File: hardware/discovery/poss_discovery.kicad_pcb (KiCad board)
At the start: 2 copper layers, 96.5 x 66 mm, 118 parts, among them CON1 USB-MICRO-B, SW1 SW_PUSH, SW10 SW_PUSH, SW11 SW_PUSH, SW12 SW_PUSH, SW13 SW_PUSH, SW14 SW_PUSH, SW15 SW_PUSH, SW16 SW_PUSH, SW18 SW_PUSH, SW19 SW_PUSH, SW2 SW_PUSH, SW20 SW_PUSH, SW21 SW_PUSH, SW22 SW_PUSH, SW3 SW_PUSH, SW4 SW_PUSH, SW5 SW_PUSH, SW6 SW_PUSH, SW7 SW_PUSH, SW8 SW_PUSH, SW9 SW_PUSH, U10 STM32_SWD_Connector, U2 MCP73831, U3 BD33IA5, U4 STM32F407VG, U5 SGTL5000, U6 encoder_and_switch, U7 encoder_and_switch, U8 MOLEX_microSD_47219-2001, U9 SSD1306, X1 CRYSTAL

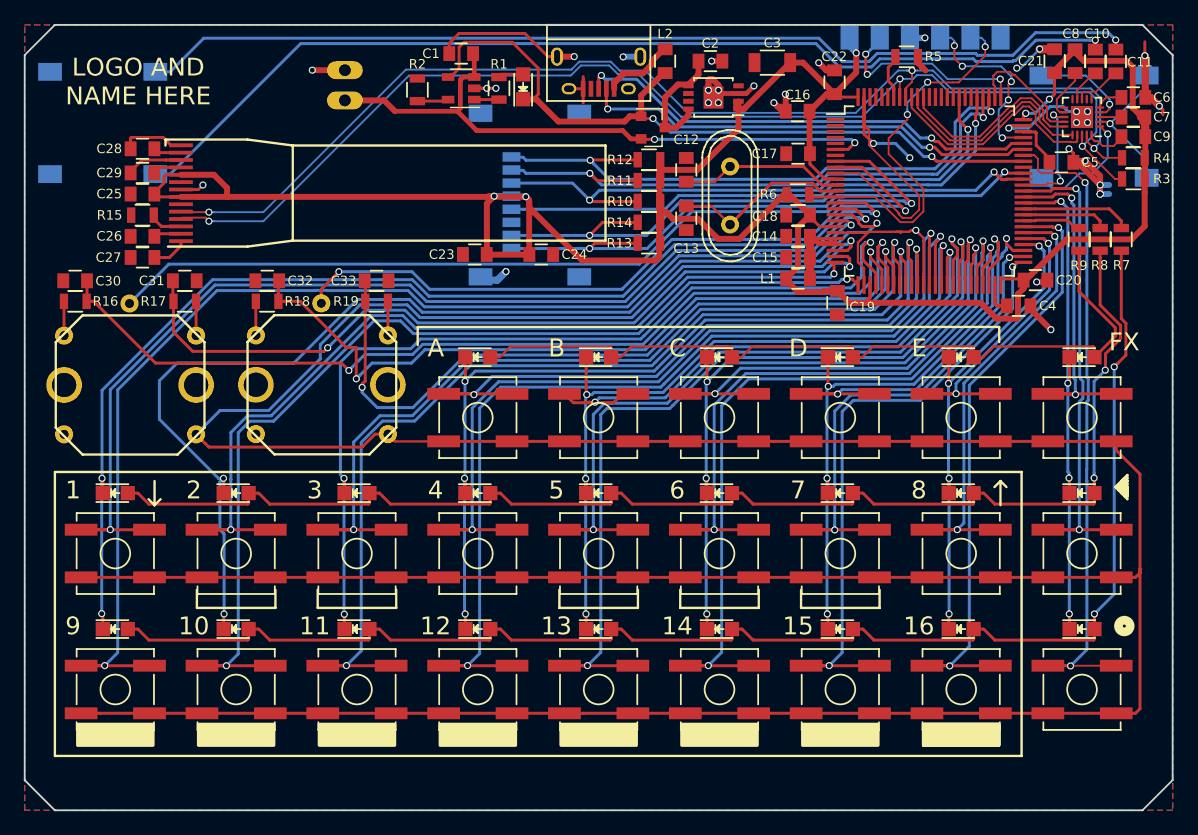
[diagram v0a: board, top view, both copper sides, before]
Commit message: Discovery: Restart from RevA
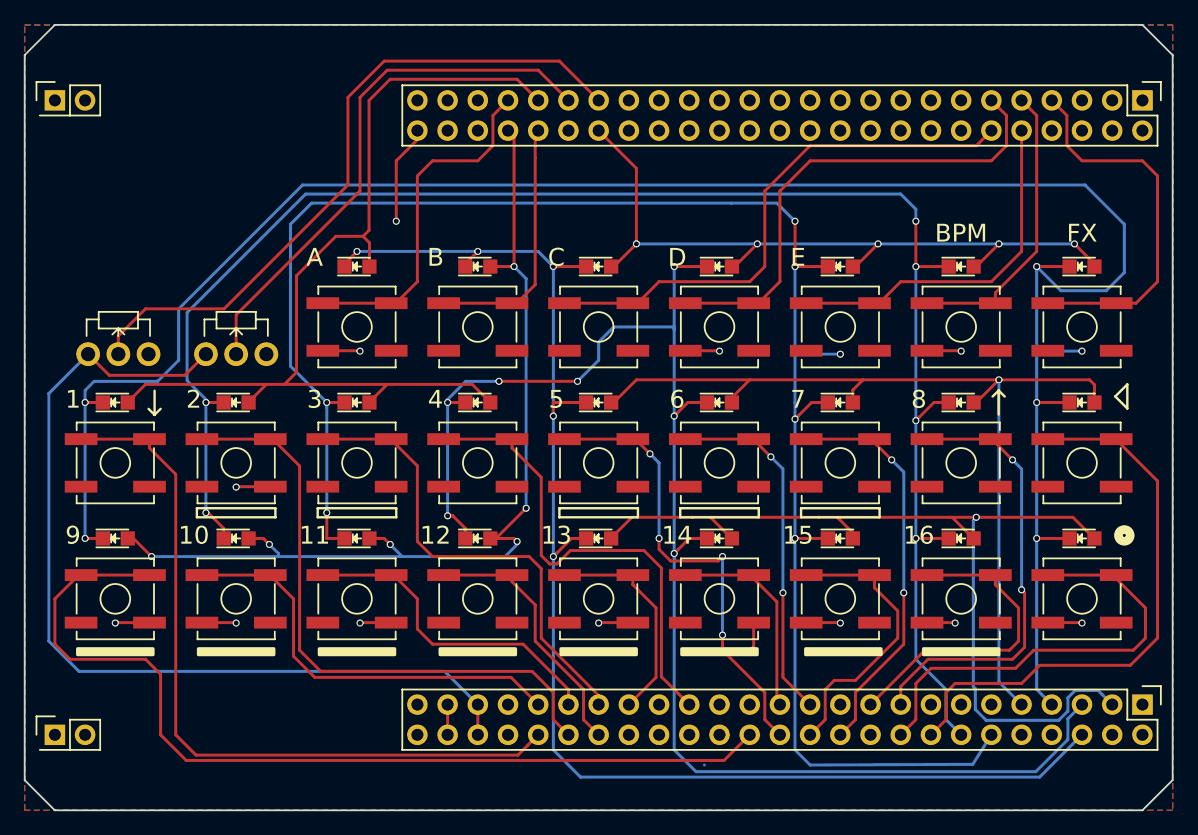
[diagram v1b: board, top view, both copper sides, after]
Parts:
- removed BAT1: LED, LEDs:LED_0805
- removed BT1: BATTERY, Connect:PINHEAD1-2
- removed C1, C25, C26, C27: 10uF, Capacitors_SMD:C_0805
- removed C10, C11, C14, C28, C29: 1uF, Capacitors_SMD:C_0805
- removed C12, C13: C, Capacitors_SMD:C_0805
- removed C15, C17, C18, C19, C20, C21, C22, C23, C6, C7, C8, C9: 0.1uF, Capacitors_SMD:C_0805
- removed C16, C24: 22uF, Capacitors_SMD:C_0805
- removed C2: 4.7uF, Capacitors_SMD:C_0805
- removed C3: 47uF, Capacitors_SMD:C_1206
- removed C30, C31, C32, C33: 0,1uF, Capacitors_SMD:C_0805
- removed C4, C5: 2.2uF, Capacitors_SMD:C_0805
- removed CON1: USB-MICRO-B, Connect:USB_Micro-B
- removed D27: DOUBLE_SCH_KCOM_PMEG2005CT, TO_SOT_Packages_SMD:SOT-23
- removed HP_OUT1, LINE_IN1: 3.5_audio_jack, stm32f4-disco:lumberg_3.5_audio_jack_1503_02
- removed L1, L2: 15Ohm, Capacitors_SMD:C_0805
- removed R1: 1K, Resistors_SMD:R_0805
- removed R10, R11, R12, R13, R14, R2, R3, R4, R5, R6: 10K, Resistors_SMD:R_0805
- removed R15, R7, R8, R9: R, Resistors_SMD:R_0805
- removed R16, R17, R18, R19: 27K, Resistors_SMD:R_0805
- removed U10: STM32_SWD_Connector, stm32f4-disco:STM32_SWD_Connector_SMD
- removed U2: MCP73831, TO_SOT_Packages_SMD:SOT-23-5
- removed U3: BD33IA5, Housings_SSOP:MSOP-8-1EP_3x3mm_Pitch0.65mm
- removed U4: STM32F407VG, Housings_QFP:LQFP-100_14x14mm_Pitch0.5mm
- removed U5: SGTL5000, Housings_DFN_QFN:UQFN-20-1EP_3x3mm_Pitch0.4mm
- removed U6, U7: encoder_and_switch, stm32f4-disco:encoder_EC12D
- removed U8: MOLEX_microSD_47219-2001, stm32f4-disco:MOLEX_microSD_47219-2001
- removed U9: SSD1306, stm32f4-disco:MIDAS_MCOT096016AV_OLED
- removed X1: CRYSTAL, Crystals:Crystal_HC49-U_Vertical
- added D19: LED, LEDs:LED_0805, F.Cu at (97.8, 110.5)
- added J1: HEADER_2, Pin_Headers:Pin_Header_Straight_2x01, F.Cu at (82.5, 85.1)
- added J2: HEADER_25x2, Pin_Headers:Pin_Header_Straight_2x25, F.Cu at (174.0, 85.1)
- added J3: HEADER_25x2, Pin_Headers:Pin_Header_Straight_2x25, F.Cu at (174.0, 135.9)
- added J5: HEADER_2, Pin_Headers:Pin_Header_Straight_2x01, F.Cu at (82.5, 138.4)
- added RV1: POT, Potentiometers:Potentiometer_WirePads_Small, F.Cu at (95.2, 106.4)
- added RV2: POT, Potentiometers:Potentiometer_WirePads_Small, F.Cu at (85.3, 106.4)
- added SW17: SW_PUSH, Buttons_Switches_SMD:SW_SPST_B3SL-1002P, F.Cu at (108.0, 104.1)
- moved D25 82.7 mm to (87.6, 121.9)
- moved D10 81.6 mm to (168.9, 110.5)
- moved D24 62.8 mm to (97.8, 121.9)
- moved D18 61.4 mm to (108.0, 110.5)
- moved D16 44.9 mm to (108.0, 99.1)
- moved D23 43.4 mm to (108.0, 121.9)
- moved D1 41.3 mm to (128.3, 121.9)
- moved D17 41.3 mm to (118.1, 110.5)
- moved D2 41.3 mm to (138.4, 121.9)
- moved D3 41.3 mm to (148.6, 121.9)
- moved D4 41.3 mm to (158.8, 121.9)
- moved D5 41.3 mm to (168.9, 121.9)
- moved D11 35.9 mm to (128.3, 99.1)
- moved D12 35.9 mm to (138.4, 99.1)
- moved D13 35.9 mm to (148.6, 99.1)
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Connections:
- net WAKEUP renamed /GND
- D1 pad 1: COL1 -> /PC9
- D1 pad 2: Net-(D1-Pad2) -> /COL1
- D10 pad 1: COL1 -> /PA8
- D10 pad 2: Net-(D10-Pad2) -> /COL2
- D11 pad 1: COL2 -> /PC9
- D11 pad 2: Net-(D10-Pad2) -> /COL3
- D12 pad 1: COL3 -> /PC8
- D12 pad 2: Net-(D10-Pad2) -> /COL3
- D13 pad 1: COL4 -> /PA15
- D13 pad 2: Net-(D10-Pad2) -> /COL3
- D14 pad 1: COL5 -> /PC11
- D14 pad 2: Net-(D10-Pad2) -> /COL3
- D15 pad 1: COL6 -> /PA8
- D15 pad 2: Net-(D10-Pad2) -> /COL3
- D16 pad 1: COL7 -> /PC9
- D16 pad 2: Net-(D10-Pad2) -> /COL4
- D17 pad 1: COL8 -> /PC8
- D17 pad 2: Net-(D10-Pad2) -> /COL4
- D18 pad 1: COL9 -> /PA15
- D18 pad 2: Net-(D10-Pad2) -> /COL4
- D2 pad 1: COL2 -> /PC8
- D2 pad 2: Net-(D1-Pad2) -> /COL1
- D20 pad 1: COL4 -> /PA8
- D20 pad 2: Net-(D20-Pad2) -> /COL4
- D21 pad 1: COL5 -> /PC9
- D21 pad 2: Net-(D20-Pad2) -> /COL5
- D22 pad 1: COL6 -> /PC8
- D22 pad 2: Net-(D20-Pad2) -> /COL5
- D23 pad 1: COL7 -> /PA15
- D23 pad 2: Net-(D20-Pad2) -> /COL5
- D24 pad 1: COL8 -> /PC11
- D24 pad 2: Net-(D20-Pad2) -> /COL5
- D25 pad 1: COL9 -> /PA8
- D25 pad 2: Net-(D20-Pad2) -> /COL5
- D3 pad 1: COL3 -> /PA15
- D3 pad 2: Net-(D1-Pad2) -> /COL1
- D4 pad 1: COL4 -> /PC11
- D4 pad 2: Net-(D1-Pad2) -> /COL1
- D5 pad 1: COL5 -> /PA8
- D5 pad 2: Net-(D1-Pad2) -> /COL1
- D6 pad 1: COL6 -> /PC9
- D6 pad 2: Net-(D1-Pad2) -> /COL2
- D7 pad 1: COL7 -> /PC8
- D7 pad 2: Net-(D1-Pad2) -> /COL2
- D8 pad 1: COL8 -> /PA15
- D8 pad 2: Net-(D1-Pad2) -> /COL2
- D9 pad 1: COL9 -> /PC11
- D9 pad 2: Net-(D1-Pad2) -> /COL2
- Play1 pad 1: Play -> /PD0
- Play2 pad 1: FX -> /FX
- SW1 pad 1: B1 -> /B1
- SW10 pad 1: B10 -> /B10
- SW11 pad 1: B11 -> /B11
- SW12 pad 1: B12 -> /B12
- SW13 pad 1: B13 -> /B13
- SW14 pad 1: B14 -> /B14
- SW15 pad 1: B15 -> /B15
- SW16 pad 1: B16 -> /B16
- SW18 pad 1: BA -> /BF2
- SW19 pad 1: BB -> /BF3
- SW2 pad 1: B2 -> /B2
- SW20 pad 1: BC -> /BF4
- SW21 pad 1: BD -> /BF5
- SW22 pad 1: BE -> /BPM
- SW3 pad 1: B3 -> /B3
- SW4 pad 1: B4 -> /B4
- SW5 pad 1: B5 -> /B5
- SW6 pad 1: B6 -> /B6
- SW7 pad 1: B7 -> /B7
- SW8 pad 1: B8 -> /B8
- SW9 pad 1: B9 -> /B9
- Write1 pad 1: Write -> /PD2
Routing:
- net /GND: track 346.7 -> 42.0 mm, vias 1 -> 13
- net 3V3: track 214.2 -> 0.00 mm, vias 5 -> 0
- net /PA8: track 0.00 -> 172.4 mm, vias 0 -> 5
- net /PA15: track 0.00 -> 146.8 mm, vias 0 -> 6
- net /PC11: track 0.00 -> 142.5 mm, vias 0 -> 6
- net /PC8: track 0.00 -> 125.1 mm, vias 0 -> 7
- net Net-(D1-Pad2): track 124.5 -> 0.00 mm, vias 2 -> 0
- net GND: track 120.9 -> 0.00 mm, vias 36 -> 0
- net /PC9: track 0.00 -> 118.0 mm, vias 0 -> 5
- net Net-(D10-Pad2): track 113.4 -> 0.00 mm, vias 2 -> 0
- net B9: track 101.4 -> 0.00 mm, vias 2 -> 0
- net Audio_SDA: track 98.1 -> 0.00 mm, vias 3 -> 0
- net COL1: track 97.8 -> 0.00 mm, vias 3 -> 0
- net Audio_SCL: track 97.8 -> 0.00 mm, vias 3 -> 0
- net COL2: track 95.7 -> 0.00 mm, vias 3 -> 0
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- added copper zone on B.Cu, net /GND
- added copper zone on F.Cu, net /GND
- removed copper zone on B.Cu, net GND
- removed copper zone on F.Cu, net GND
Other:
- net class DAC_traces removed
- net class power removed
- rule trace_min: 0.16 -> 0.2
- board text added: "BPM"
- board text removed: "GND"
- board text removed: "IN"
- board text removed: "LOGO AND NAME HERE"
- board text removed: "NRST"
- board text removed: "OUT"
- board text removed: "RevB"
- board text removed: "SWCLK"
- board text removed: "SWDIO"
- board text removed: "SWO"
- board text removed: "VCC"
